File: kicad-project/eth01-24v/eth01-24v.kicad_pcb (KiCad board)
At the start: 2 copper layers, 4 parts, among them U1 WT32-ETH01, U2 XL-6009-ADJ

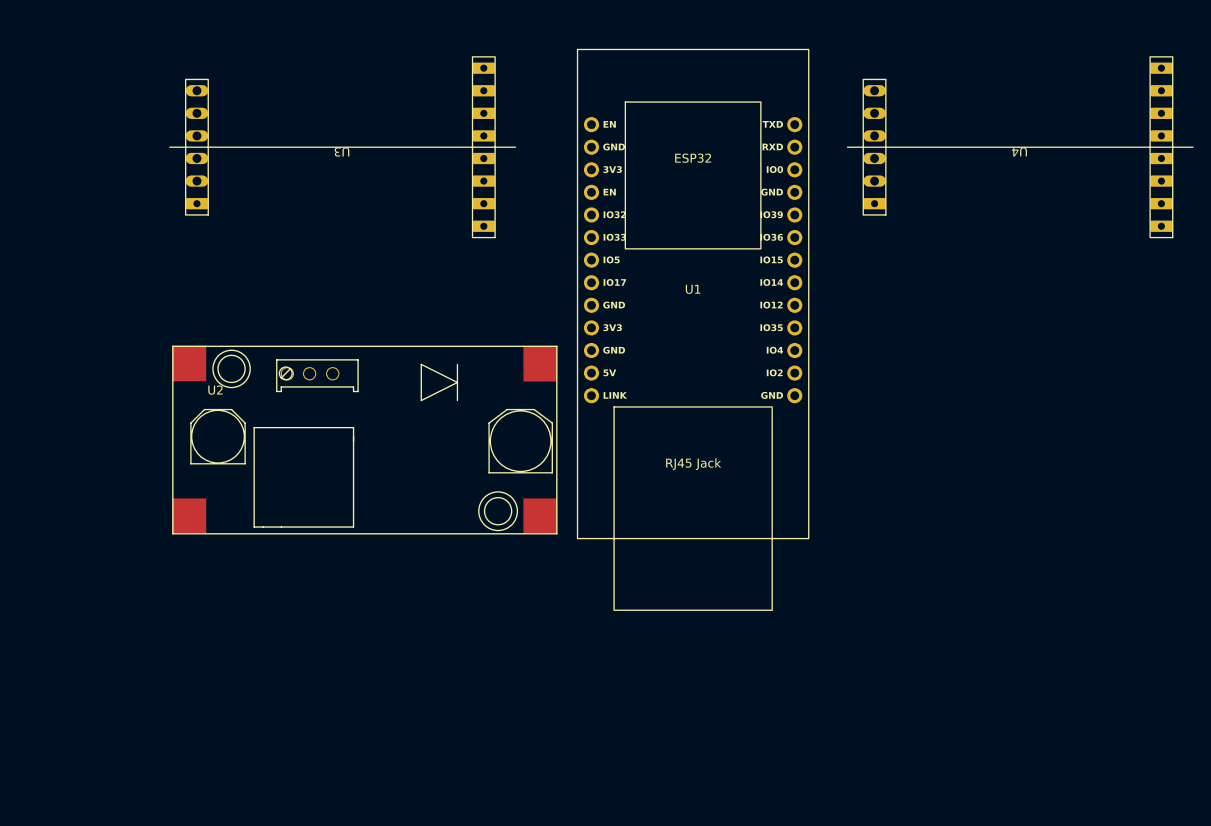
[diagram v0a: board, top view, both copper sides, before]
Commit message: ajout photos et première version pcb
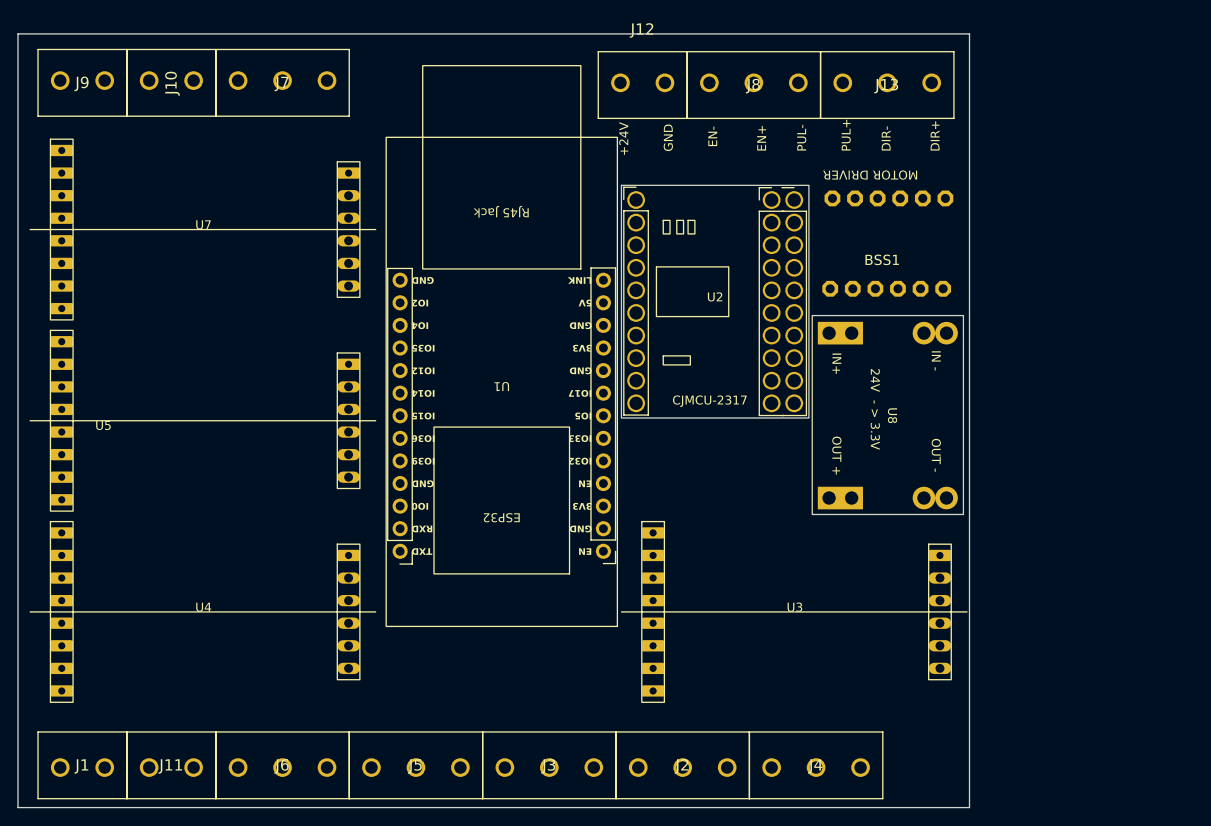
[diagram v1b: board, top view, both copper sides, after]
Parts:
- added BSS1: ~, WT32-ETH01:BSS138, F.Cu at (175.4, 89.6)
- added J1: KF301-2P, WT32-ETH01:KF3012P, F.Cu at (82.5, 148.5)
- added J10: KF301-2P, WT32-ETH01:KF3012P, F.Cu at (97.5, 71.2)
- added J11: KF301-2P, WT32-ETH01:KF3012P, F.Cu at (92.5, 148.5)
- added J12: KF301-2P, WT32-ETH01:KF3012P, F.Cu at (150.5, 71.5)
- added J13: KF301-3P, WT32-ETH01:KF3013P, F.Cu at (180.5, 71.5)
- added J2: KF301-3P, WT32-ETH01:KF3013P, F.Cu at (147.5, 148.5)
- added J3: KF301-3P, WT32-ETH01:KF3013P, F.Cu at (132.5, 148.5)
- added J4: KF301-3P, WT32-ETH01:KF3013P, F.Cu at (162.5, 148.5)
- added J5: KF301-3P, WT32-ETH01:KF3013P, F.Cu at (117.5, 148.5)
- added J6: KF301-3P, WT32-ETH01:KF3013P, F.Cu at (102.5, 148.5)
- added J7: KF301-3P, WT32-ETH01:KF3013P, F.Cu at (112.5, 71.2)
- added J8: KF301-3P, WT32-ETH01:KF3013P, F.Cu at (165.5, 71.5)
- added J9: KF301-2P, WT32-ETH01:KF3012P, F.Cu at (87.5, 71.2)
- added U5: ~, WT32-ETH01:OP71A04, F.Cu at (79.1, 109.5)
- added U7: ~, WT32-ETH01:OP71A04, F.Cu at (79.1, 88.0)
- added U8: ~, WT32-ETH01:MP1584_AIO, F.Cu at (175.6, 108.9)
- U2: value XL-6009-ADJ -> ~; footprint esp32-24v-io:XL6009_module_SMT -> WT32-ETH01:MCP23017
- moved U4 140.8 mm to (79.1, 131.0), turned to 0 degrees
- moved U3 53.6 mm to (145.6, 131.0), turned to 0 degrees
- moved U2 31.6 mm to (156.2, 96.1)
- moved U1 23.7 mm to (132.2, 105.1), turned to 180 degrees
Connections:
- U1 pad 10: Net-(U4-Vcc) -> 3.3V
- U1 pad 12: Net-(U1-5V) -> 5V
- U1 pad 16: unconnected-(U1-IO4/ADC2_CH0/TCH0-Pad16) -> Net-(BSS1-LV3)
- U1 pad 19: Net-(U1-IO14/ADC2_CH6/TCH6) -> Net-(BSS1-LV2)
- U1 pad 20: Net-(U1-IO15/ADC2_CH3/TCH3) -> Net-(BSS1-LV1)
- U1 pad 21: Net-(U1-IO36/ADC1_CH0/INPUT_ONLY) -> /InterruptA
- U1 pad 22: Net-(U1-IO39/ADC1_CH3/INPUT_ONLY) -> /InteruptB
- U1 pad 23: unconnected-(U1-GND-Pad23) -> GND
- U1 pad 3: Net-(U4-Vcc) -> 3.3V
- U1 pad 5: Net-(U1-IO32/ADC1_CH4/TCH9) -> /SCL
- U1 pad 6: Net-(U1-IO33/ADC1_CH5/TCH8) -> /SDA
- U1 pad 7: Net-(U1-IO5/BOOT_FLOAT) -> unconnected-(U1-IO5/BOOT_FLOAT-Pad7)
- U1 pad 8: Net-(U1-IO17/UART2_TX) -> unconnected-(U1-IO17/UART2_TX-Pad8)
- U2 pad 1: +24V -> unconnected-(U2-A2-Pad1)
- U2 pad 2: GND -> unconnected-(U2-A1-Pad2)
- U2 pad 3: Net-(U1-5V) -> unconnected-(U2-A0-Pad3)
- U2 pad 4: GND -> unconnected-(U2-RESET-Pad4)
- U3 pad 1: Net-(U1-IO32/ADC1_CH4/TCH9) -> Net-(U3-1+)
- U3 pad 11: OUT1 -> Net-(U2-B3)
- U3 pad 12: OUT2 -> Net-(U2-B2)
- U3 pad 13: OUT3 -> Net-(U2-B1)
- U3 pad 14: OUT4 -> Net-(U2-B0)
- U3 pad 3: Net-(U1-IO33/ADC1_CH5/TCH8) -> Net-(U3-2+)
- U3 pad 5: Net-(U1-IO5/BOOT_FLOAT) -> Net-(U3-3+)
- U3 pad 7: Net-(U1-IO17/UART2_TX) -> Net-(U3-4+)
- U3 pad 9: +24V -> 3.3V
- U4 pad 1: IN1-24V -> /E-STOP
- U4 pad 11: Net-(U1-IO39/ADC1_CH3/INPUT_ONLY) -> Net-(U2-B7)
- U4 pad 12: Net-(U1-IO36/ADC1_CH0/INPUT_ONLY) -> Net-(U2-B6)
- U4 pad 13: Net-(U1-IO15/ADC2_CH3/TCH3) -> Net-(U2-B5)
- U4 pad 14: Net-(U1-IO14/ADC2_CH6/TCH6) -> Net-(U2-B4)
- U4 pad 3: IN2-24V -> /SIGNAL
- U4 pad 5: IN3-24V -> Net-(U4-3+)
- U4 pad 7: IN4-24V -> Net-(U4-4+)
- U4 pad 9: Net-(U4-Vcc) -> 3.3V
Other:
- board outline added: 107 x 87 mm
- board text added: "+24V"
- board text added: "DIR+"
- board text added: "DIR-"
- board text added: "EN+"
- board text added: "EN-"
- board text added: "GND"
- board text added: "MOTOR DRIVER"
- board text added: "PUL+"
- board text added: "PUL-"
